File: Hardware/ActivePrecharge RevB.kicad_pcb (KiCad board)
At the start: 2 copper layers, 98.4 x 58.9 mm, 93 parts, among them IC1 AMC1350DWVR, IC2 AMC1350DWVR, IC3 ZXRE160AET5TA, U1 LT1963AEST-3.3#TRPBF, U2 TLV9001IDBVR, U3 TLV9001IDBVR

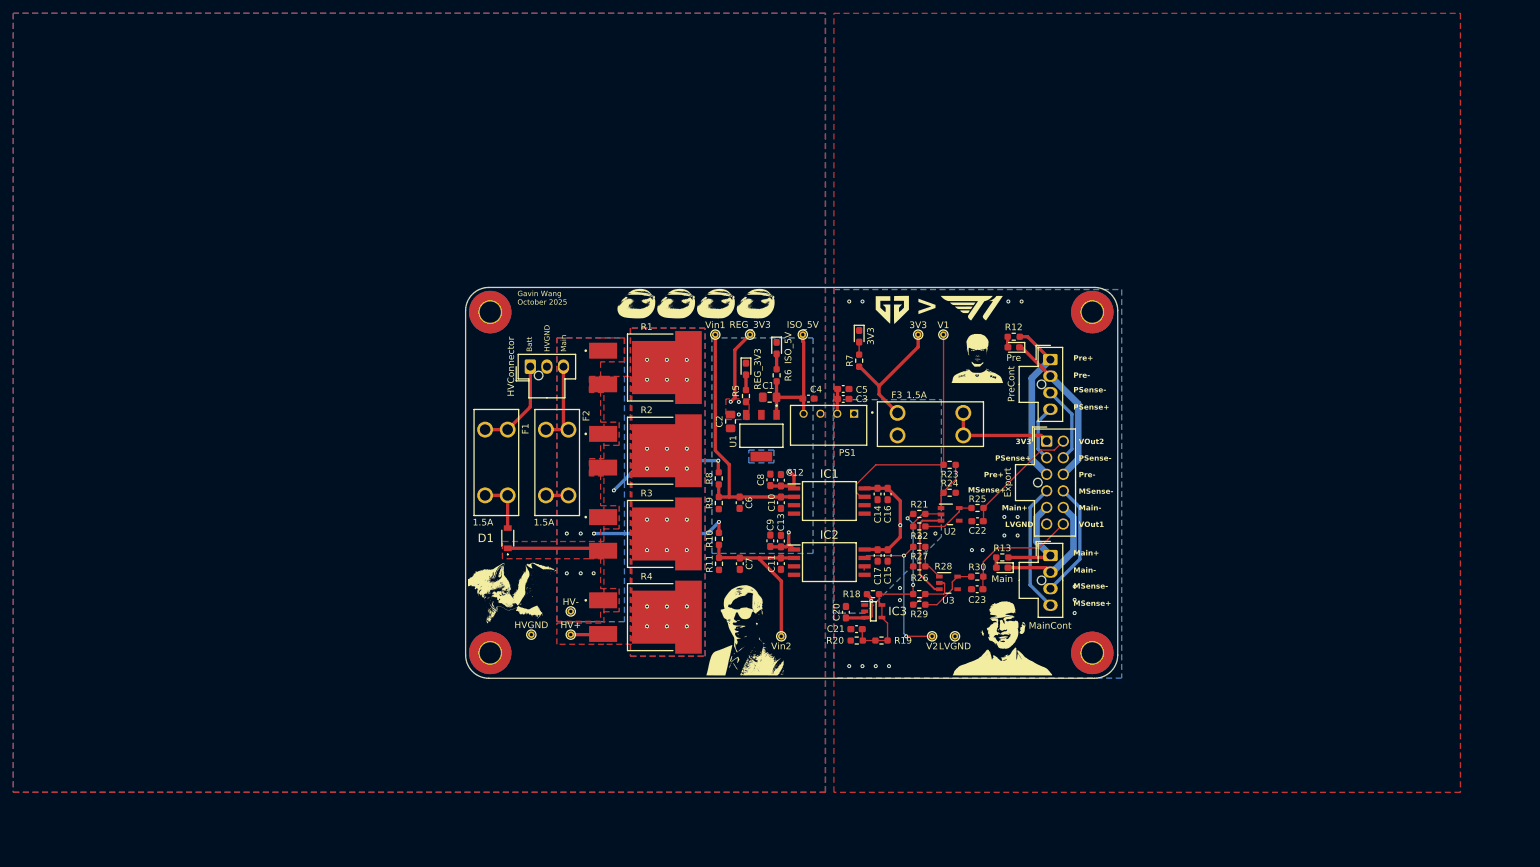
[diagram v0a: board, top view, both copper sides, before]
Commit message: Fixed this shit finally im free
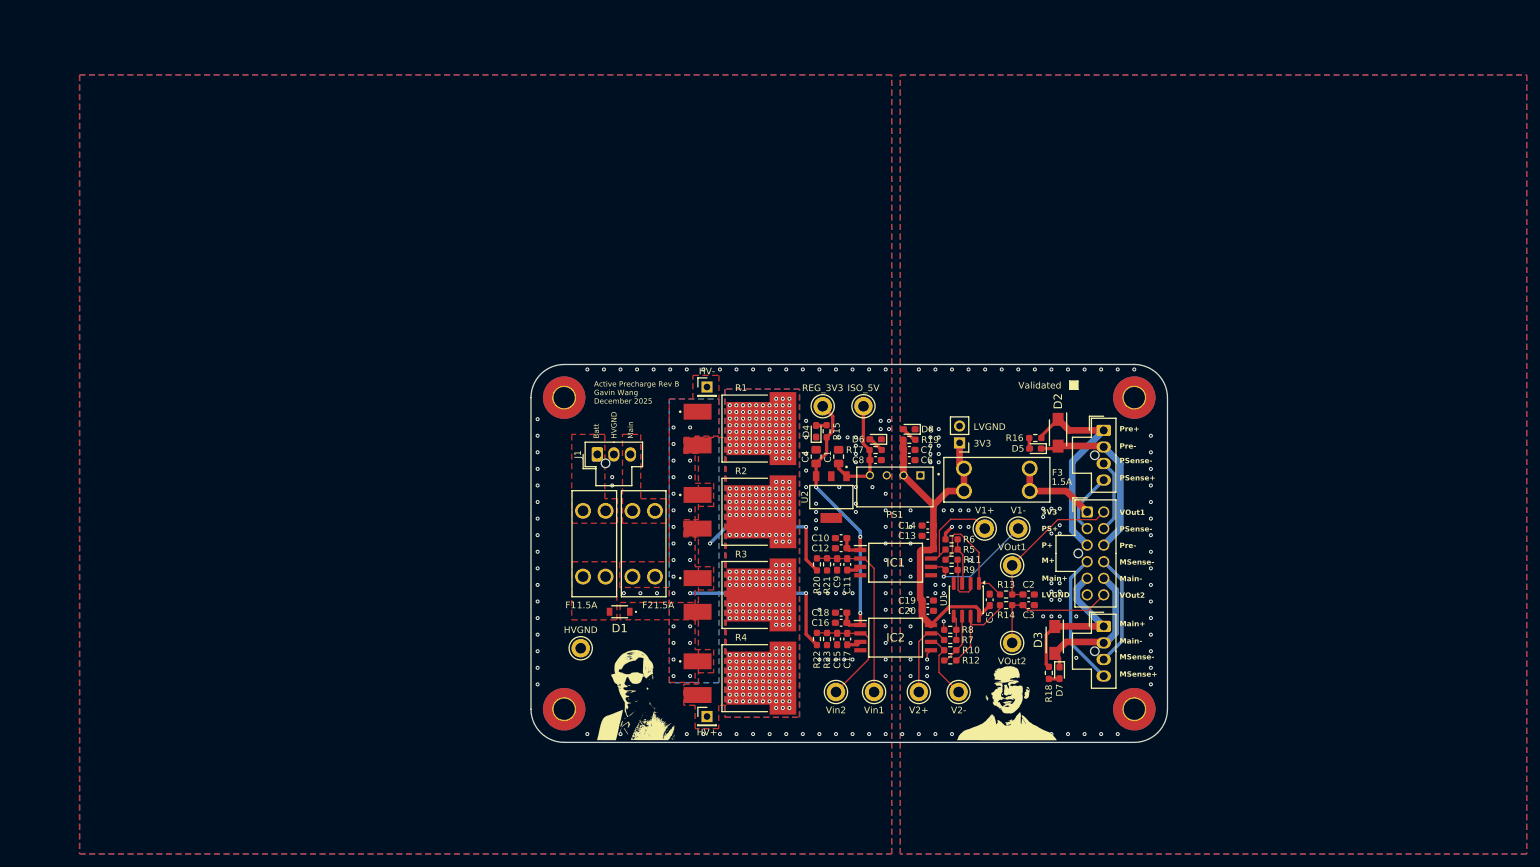
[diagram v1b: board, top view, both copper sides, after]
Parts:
- removed 3V3: 3V3, TestPoint:TestPoint_THTPad_D1.0mm_Drill0.5mm
- removed 3V3, Main, Pre: LED, LED_SMD:LED_0603_1608Metric_Pad1.05x0.95mm_HandSolder
- removed C21: 0.47uF, Capacitor_SMD:C_0603_1608Metric_Pad1.08x0.95mm_HandSolder
- removed C22, C23: 10nF, Capacitor_SMD:C_0603_1608Metric_Pad1.08x0.95mm_HandSolder
- removed Export: ExportConnector, Connector_Molex:Molex_Nano-Fit_105310-xx12_2x06_P2.50mm_Vertical
- removed the G*** at (164.5, 63.0)
- removed the G*** at (177.0, 70.6)
- removed the G*** at (176.5, 63.0)
- removed the G*** at (181.1, 111.8)
- removed the G*** at (144.0, 62.6)
- removed the G*** at (138.0, 62.6)
- removed the G*** at (126.0, 62.6)
- removed the G*** at (108.0, 106.1)
- removed the G*** at (132.0, 62.6)
- removed the HV+ at (116.0, 112.2)
- removed the HV- at (116.0, 108.8)
- removed HVConnector: HVConnector, Connector_Molex:Molex_Nano-Fit_105309-xx03_1x03_P2.50mm_Vertical
- removed the HVGND at (110.0, 112.2)
- removed IC3: ZXRE160AET5TA, ActivePrecharge-RevB:SOT95P280X100-5N
- removed the ISO_5V at (151.0, 67.0)
- removed the ISO_5V at (147.1, 69.0)
- removed LVGND: LVGND, TestPoint:TestPoint_THTPad_D1.0mm_Drill0.5mm
- removed MainCont: MainContactor, Connector_Molex:Molex_Nano-Fit_105309-xx04_1x04_P2.50mm_Vertical
- removed PreCont: PrechargeContactor, Connector_Molex:Molex_Nano-Fit_105309-xx04_1x04_P2.50mm_Vertical
- removed R24, R28, R29: 15k, Resistor_SMD:R_0603_1608Metric_Pad0.98x0.95mm_HandSolder
- removed R25, R30: 10, Resistor_SMD:R_0603_1608Metric_Pad0.98x0.95mm_HandSolder
- removed R26, R27: 2.49k, Resistor_SMD:R_0603_1608Metric_Pad0.98x0.95mm_HandSolder
- removed the REG_3V3 at (142.4, 72.2)
- removed the REG_3V3 at (143.1, 67.0)
- removed U3: TLV9001IDBVR, ActivePrecharge-RevB:DBV0005A_N
- removed V1: V1, TestPoint:TestPoint_THTPad_D1.0mm_Drill0.5mm
- removed V2: V2, TestPoint:TestPoint_THTPad_D1.0mm_Drill0.5mm
- added C18: 1uF, Capacitor_SMD:C_0603_1608Metric_Pad1.08x0.95mm_HandSolder, F.Cu at (156.8, 108.9)
- added C19: 1uF, Capacitor_SMD:C_0603_1608Metric_Pad1.08x0.95mm_HandSolder, F.Cu at (169.8, 107.1)
- added D2: VSSAF522-M3/H, UTSVT-Passives:SODFL5026X125N, F.Cu at (189.5, 81.8)
- added D3: VSSAF522-M3/H, UTSVT-Passives:SODFL5026X125N, F.Cu at (189.0, 113.0)
- added D4: LED, LED_SMD:LED_0603_1608Metric_Pad1.05x0.95mm_HandSolder, F.Cu at (153.0, 81.6)
- added D5: LED, LED_SMD:LED_0603_1608Metric_Pad1.05x0.95mm_HandSolder, F.Cu at (186.1, 84.2)
- added D6: LED, LED_SMD:LED_0603_1608Metric_Pad1.05x0.95mm_HandSolder, F.Cu at (162.0, 82.8)
- added D7: LED, LED_SMD:LED_0603_1608Metric_Pad1.05x0.95mm_HandSolder, F.Cu at (189.7, 118.0)
- added D8: LED, LED_SMD:LED_0603_1608Metric_Pad1.05x0.95mm_HandSolder, F.Cu at (167.1, 81.3)
- added G***: LOGO, LOGO, F.Cu at (181.8, 121.6)
- added G***: LOGO, LOGO, B.Cu at (183.0, 79.0)
- added HV+: Conn_01x01_Pin, Connector_PinHeader_2.54mm:PinHeader_1x01_P2.54mm_Vertical, F.Cu at (136.6, 124.6)
- added HV-: Conn_01x01_Pin, Connector_PinHeader_2.54mm:PinHeader_1x01_P2.54mm_Vertical, F.Cu at (136.6, 74.9)
- added HVGND: HVGND, TestPoint:TestPoint_Keystone_5005-5009_Compact, F.Cu at (117.5, 114.3)
- added ISO_5V: ISO_5V, TestPoint:TestPoint_Keystone_5005-5009_Compact, F.Cu at (160.2, 77.8)
- added J1: HVConnector, Connector_Molex:Molex_Nano-Fit_105309-xx03_1x03_P2.50mm_Vertical, F.Cu at (120.0, 85.1)
- added J2: PrechargeContactor, Connector_Molex:Molex_Nano-Fit_105309-xx04_1x04_P2.50mm_Vertical, F.Cu at (196.4, 81.4)
- added J3: MainContactor, Connector_Molex:Molex_Nano-Fit_105309-xx04_1x04_P2.50mm_Vertical, F.Cu at (196.4, 111.0)
- added J4: ExportConnector, Connector_Molex:Molex_Nano-Fit_105310-xx12_2x06_P2.50mm_Vertical, F.Cu at (193.9, 93.8)
- added J7: Conn_01x02_Pin, Connector_PinHeader_2.54mm:PinHeader_1x02_P2.54mm_Vertical, F.Cu at (174.6, 83.3)
- added R14: 10, Resistor_SMD:R_0603_1608Metric_Pad0.98x0.95mm_HandSolder, F.Cu at (181.7, 107.8)
- added R15: 1k, Resistor_SMD:R_0603_1608Metric_Pad0.98x0.95mm_HandSolder, F.Cu at (154.6, 81.6)
- added R16: 10k, Resistor_SMD:R_0603_1608Metric_Pad0.98x0.95mm_HandSolder, F.Cu at (186.1, 82.6)
- added R17: 1k, Resistor_SMD:R_0603_1608Metric_Pad0.98x0.95mm_HandSolder, F.Cu at (162.0, 84.4)
- added REG_3V3: REG_3V3, TestPoint:TestPoint_Keystone_5005-5009_Compact, F.Cu at (154.0, 77.8)
- added V1+: V+, TestPoint:TestPoint_Keystone_5005-5009_Compact, F.Cu at (178.4, 96.2)
- added V1-: V-, TestPoint:TestPoint_Keystone_5005-5009_Compact, F.Cu at (183.5, 96.2)
- added V2+: V+, TestPoint:TestPoint_Keystone_5005-5009_Compact, F.Cu at (168.5, 120.9)
- added V2-: V-, TestPoint:TestPoint_Keystone_5005-5009_Compact, F.Cu at (174.5, 120.9)
- added VOut1: VOut1, TestPoint:TestPoint_Keystone_5005-5009_Compact, F.Cu at (182.6, 101.8)
- added VOut2: VOut2, TestPoint:TestPoint_Keystone_5005-5009_Compact, F.Cu at (182.6, 113.5)
- C10: value 1nF -> 100nF
- C14: value 1uF -> 100nF
- C17: value 100nF -> 1nF
- C2: value 10uF -> 10nF; footprint Capacitor_SMD:C_0805_2012Metric_Pad1.18x1.45mm_HandSolder -> Capacitor_SMD:C_0603_1608Metric_Pad1.08x0.95mm_HandSolder
- C3: value 1uF -> 10nF
- C4: value 1uF -> 10uF; footprint Capacitor_SMD:C_0603_1608Metric_Pad1.08x0.95mm_HandSolder -> Capacitor_SMD:C_0805_2012Metric_Pad1.18x1.45mm_HandSolder
- C8, C9: value 100nF -> 1uF
- R10, R8: value 100k -> 10k
- R11, R9: value 2.49k -> 10k
- R12, R18, R5, R6, R7: value 1k -> 10k
- R13: value 1k -> 10
- R19: value 5.1k -> 1k
- R20, R22: value 15k -> 100k
- U1: value LT1963AEST-3.3#TRPBF -> TLV9002QDRQ1; footprint ActivePrecharge-RevB:VREG_LT1963AEST-3.3_TRPBF -> Package_SO:SOIC-8_3.9x4.9mm_P1.27mm
- U2: value TLV9001IDBVR -> LT1963AEST-3.3#TRPBF; footprint ActivePrecharge-RevB:DBV0005A_N -> ActivePrecharge-RevB:VREG_LT1963AEST-3.3_TRPBF
- Vin1: value Vin1 -> Vin; footprint TestPoint:TestPoint_THTPad_D1.0mm_Drill0.5mm -> TestPoint:TestPoint_Keystone_5005-5009_Compact
- Vin2: value Vin2 -> Vin; footprint TestPoint:TestPoint_THTPad_D1.0mm_Drill0.5mm -> TestPoint:TestPoint_Keystone_5005-5009_Compact
- moved LOGO2 61.1 mm to (175.1, 74.9)
- moved Vin1 59.0 mm to (161.8, 120.9)
- moved C2 52.0 mm to (185.1, 106.2), turned to 0 degrees
- moved R12 49.8 mm to (173.2, 116.1), turned to 0 degrees
- moved R7 44.3 mm to (173.2, 113.1), turned to 180 degrees
- moved C3 41.8 mm to (185.1, 107.8)
- moved R8 41.7 mm to (173.2, 111.5), turned to 0 degrees
- moved U1 39.6 mm to (175.7, 107.0)
- moved R10 38.7 mm to (173.2, 114.6), turned to 0 degrees
- moved C5 38.7 mm to (179.2, 107.0), turned to 90 degrees
- moved R5 38.7 mm to (173.4, 99.4), turned to 180 degrees
- moved R9 36.5 mm to (173.4, 102.5), turned to 180 degrees
- moved R6 36.2 mm to (173.4, 97.9), turned to 0 degrees
- moved R11 35.1 mm to (173.4, 101.0), turned to 0 degrees
- moved R23 32.1 mm to (154.7, 112.9), turned to 90 degrees
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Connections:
- net Net-(D1-A) renamed /HV+_Fused
- C10 pad 1: /Voltage_Sense/Vin1 -> REG_3V3
- C11 pad 1: /Voltage_Sense/Vin2 -> /Vin1
- C13 pad 1: REG_3V3 -> 3V3
- C13 pad 2: HVGND -> LVGND
- C15 pad 1: 3V3 -> /Vin2
- C15 pad 2: LVGND -> HVGND
- C16 pad 1: 3V3 -> REG_3V3
- C16 pad 2: LVGND -> HVGND
- C17 pad 1: 3V3 -> /Vin2
- C17 pad 2: LVGND -> HVGND
- C2 pad 1: HVGND -> /VOut1
- C2 pad 2: REG_3V3 -> LVGND
- C3 pad 1: 3V3 -> /VOut2
- C4 pad 2: ISO_5V -> REG_3V3
- C6 pad 1: /Voltage_Sense/Vin1 -> 3V3
- C6 pad 2: HVGND -> LVGND
- C7 pad 1: /Voltage_Sense/Vin2 -> 3V3
- C7 pad 2: HVGND -> LVGND
- C8 pad 1: REG_3V3 -> HVGND
- C8 pad 2: HVGND -> ISO_5V
- C9 pad 1: REG_3V3 -> /Vin1
- F1 pad 1: Net-(J1-Pin_1) -> /HV+_PreFuse
- F2 pad 1: Net-(J1-Pin_3) -> /HV-_PreFuse
- F3 pad 2: Net-(J2-Pin_1) -> /3V3_PreFuse
- IC1 pad 2: /Voltage_Sense/Vin1 -> /Vin1
- IC1 pad 6: LVGND -> /V1-
- IC1 pad 7: /Voltage_Sense/V1 -> /V1+
- IC2 pad 2: /Voltage_Sense/Vin2 -> /Vin2
- IC2 pad 6: LVGND -> /V2-
- IC2 pad 7: /Voltage_Sense/V2 -> /V2+
- R10 pad 1: /Voltage_Sense/Vin2 -> /V2-
- R10 pad 2: HV- -> Net-(U1B--)
- R11 pad 1: HVGND -> Net-(R11-Pad1)
- R11 pad 2: /Voltage_Sense/Vin2 -> Net-(U1A--)
- R12 pad 1: /Pre+ -> Net-(U1B--)
- R12 pad 2: Net-(D5-A) -> Net-(R12-Pad2)
- R13 pad 1: /Main+ -> /VOut1
- R13 pad 2: Net-(D6-A) -> Net-(R11-Pad1)
- R18 pad 1: 3V3 -> /Main+
- R18 pad 2: REG_0V8 -> Net-(D7-A)
- R19 pad 1: REG_0V8 -> 3V3
- R19 pad 2: REG_0V8 -> Net-(D8-A)
- R20 pad 1: REG_0V8 -> /Vin1
- R20 pad 2: LVGND -> HV+
- R21 pad 1: REG_0V8 -> HVGND
- R21 pad 2: Net-(U2--) -> /Vin1
- R22 pad 1: Net-(R22-Pad1) -> /Vin2
- R22 pad 2: Net-(U2--) -> HV-
- R23 pad 1: Net-(U2-+) -> HVGND
- R23 pad 2: /Voltage_Sense/V1 -> /Vin2
- R5 pad 1: REG_3V3 -> Net-(U1A-+)
- R5 pad 2: Net-(D2-A) -> /V1+
- R6 pad 1: ISO_5V -> LVGND
- R6 pad 2: Net-(D3-A) -> Net-(U1A-+)
- R7 pad 1: 3V3 -> Net-(U1B-+)
- R7 pad 2: Net-(D4-A) -> /V2+
- R8 pad 1: /Voltage_Sense/Vin1 -> LVGND
- R8 pad 2: HV+ -> Net-(U1B-+)
- R9 pad 1: HVGND -> Net-(U1A--)
- R9 pad 2: /Voltage_Sense/Vin1 -> /V1-
- U1 pad 1: ISO_5V -> Net-(R11-Pad1)
- U1 pad 2: HVGND -> Net-(U1A--)
- U1 pad 3: REG_3V3 -> Net-(U1A-+)
- U1 pad 4: HVGND -> LVGND
- U2 pad 1: Net-(U2-+) -> ISO_5V
- U2 pad 2: Net-(U2--) -> HVGND
- U2 pad 3: 3V3 -> REG_3V3
- U2 pad 4: LVGND -> HVGND
- Vin1 pad 1: /Voltage_Sense/Vin1 -> /Vin1
- Vin2 pad 1: /Voltage_Sense/Vin2 -> /Vin2
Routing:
- net /Voltage_Sense/Vin1: track 38.6 -> 0.00 mm
- net /Voltage_Sense/V1: track 36.7 -> 0.00 mm
- net REG_0V8: track 31.1 -> 0.00 mm, vias 2 -> 0
- net /Vin1: track 0.00 -> 27.9 mm
- net /Voltage_Sense/Vin2: track 26.4 -> 0.00 mm
- net /Voltage_Sense/V2: track 24.2 -> 0.00 mm, vias 2 -> 0
- net REG_3V3: track 24.1 -> 46.8 mm, vias 5 -> 3
- net /Vin2: track 0.00 -> 18.3 mm
- net Net-(R11-Pad1): track 0.00 -> 17.8 mm
- net /V1-: track 0.00 -> 17.8 mm, vias 0 -> 1
- net Net-(J2-Pin_1): track 16.3 -> 0.00 mm
- net HV+: track 38.9 -> 22.8 mm
- net /V1+: track 0.00 -> 14.7 mm
- net Net-(R12-Pad2): track 0.00 -> 14.6 mm
- net Net-(J1-Pin_1): track 14.3 -> 0.00 mm
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- added copper zone on F.Cu, net /HV+_Fused
- added copper zone on F.Cu, net /HV+_PreFuse
- added copper zone on F.Cu, net /HV-_PreFuse
- removed copper zone on B.Cu, net 3V3
- removed copper zone on B.Cu, net REG_3V3
- removed copper zone on F.Cu, net REG_3V3
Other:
- board size 98.4 x 58.9 mm -> 96 x 57 mm
- board text added: "Active Precharge Rev B Gavin Wang December 2025"
- board text added: "M+"
- board text added: "P+"
- board text added: "PS+"
- board text added: "Validated"
- board text removed: ">"
- board text removed: "Gavin Wang October 2025"
